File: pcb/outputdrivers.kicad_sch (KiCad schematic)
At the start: 15 parts, among them J7 CONTACTORS, J7 CP/PE, J7 RF, Q1 BC846, Q2 NCV8402xST, Q3 NCV8402xST, U7 74HCT04

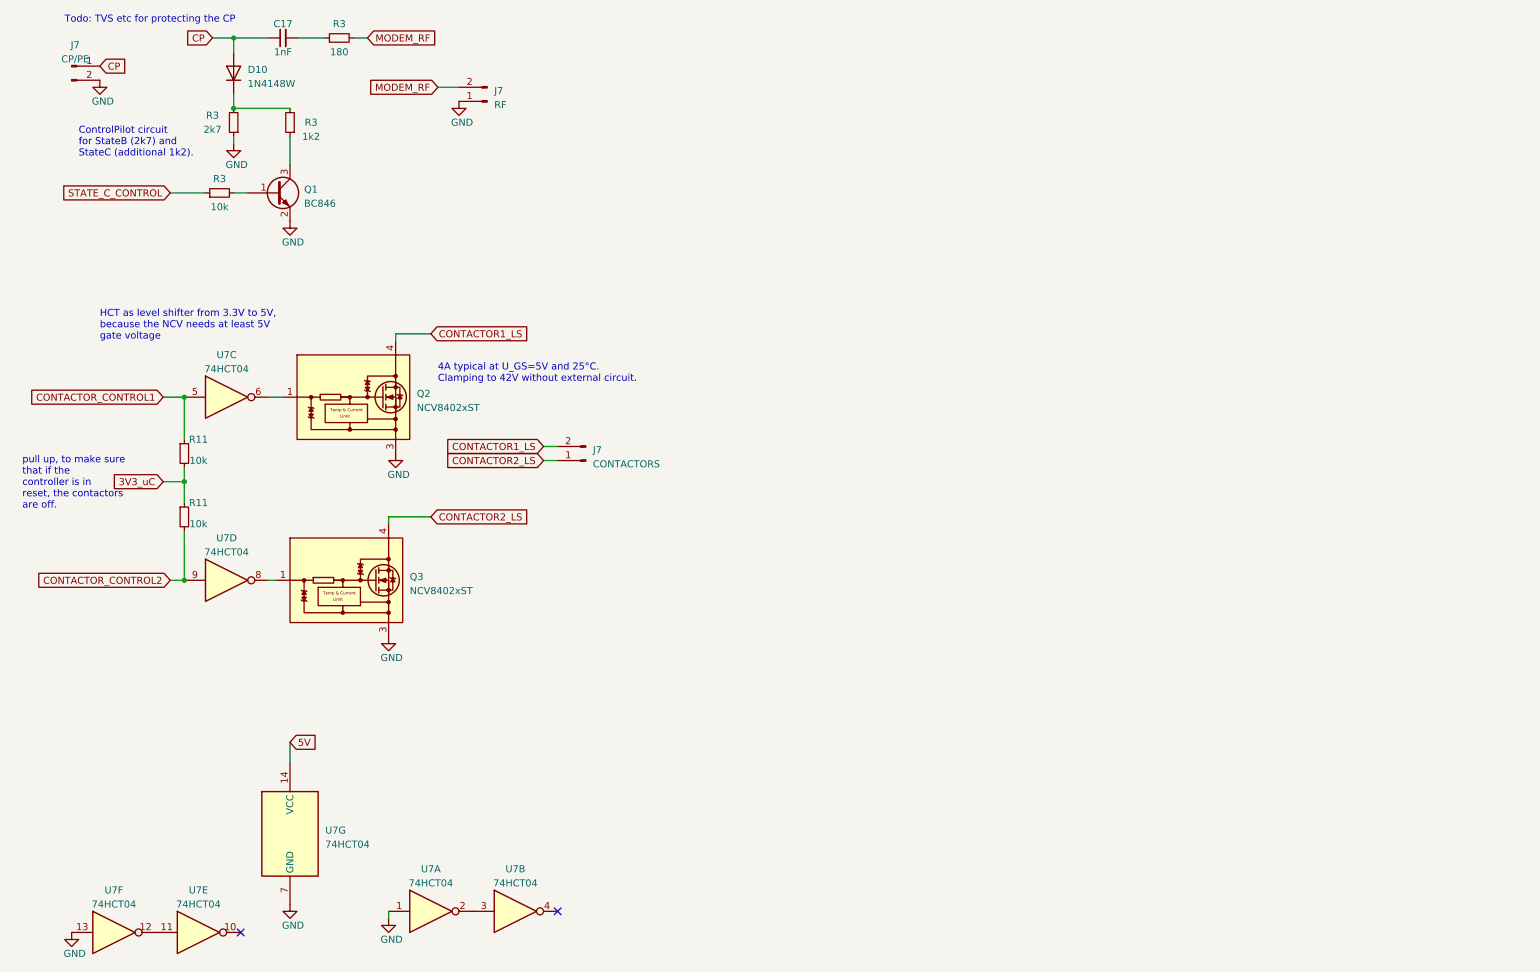
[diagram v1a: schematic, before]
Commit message: fix: divider on the stepdown. fix: non-inverted contactor drivers. fix: part number of 8MHz. add: mounting holes and spare grid. add: LIM HVDC input. docu: todo list
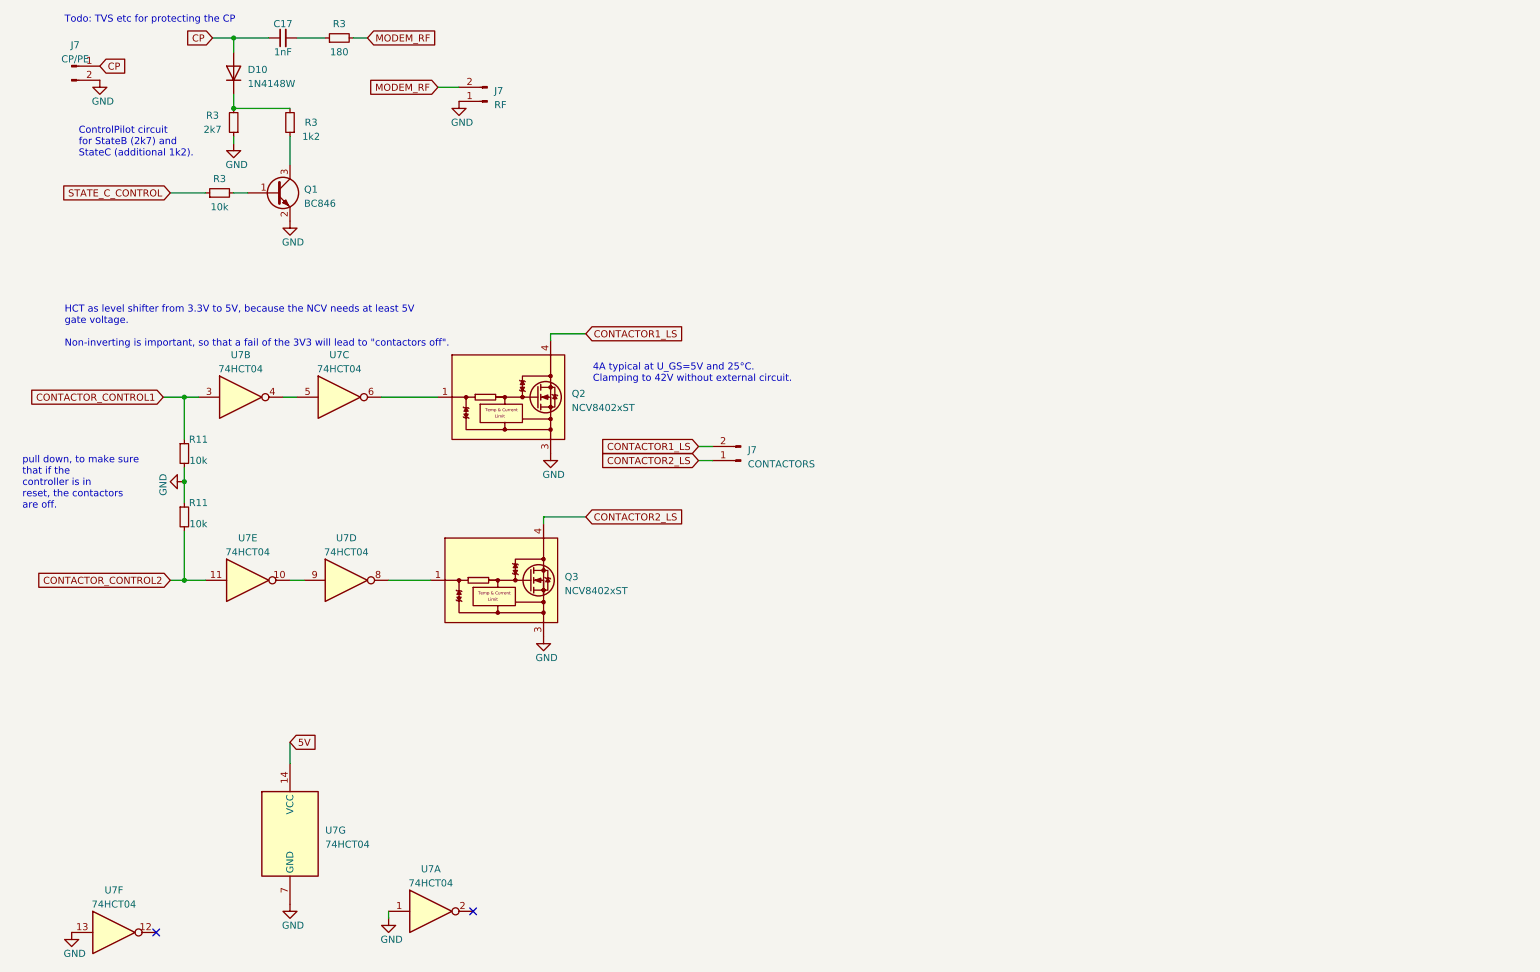
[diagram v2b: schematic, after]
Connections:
- net 3V3_uC is gone; now on net GND: R11.1, R11.2
- net CONTACTOR_CONTROL1: now also U7.3; no longer U7.5
- net CONTACTOR_CONTROL2: now also U7.11; no longer U7.9
- net at U7.2: no longer U7.3
- net at U7.12: no longer U7.11
- net at U7.10: now also U7.9
- net at U7.4: now also U7.5
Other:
- note added: "HCT as level shifter from 3.3V to 5V, because the NCV needs at least 5V gate voltage. Non-inverting is important, so that a fail of the 3V3 will lead to "contactors off"."
- note added: "pull down, to make sure that if the controller is in reset, the contactors are off."
- note removed: "HCT as level shifter from 3.3V to 5V, because the NCV needs at least 5V gate voltage"
- note removed: "pull up, to make sure that if the controller is in reset, the contactors are off."
- moved on the sheet: J7, Q2, Q3, U7B, U7C, U7D, U7E

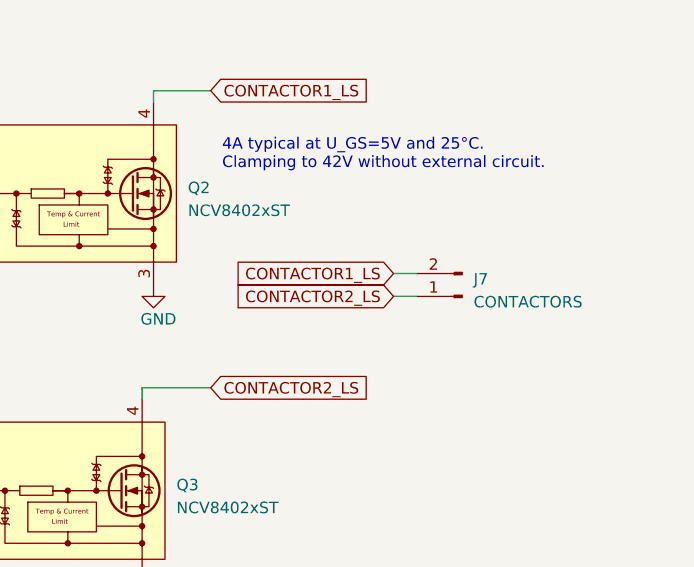
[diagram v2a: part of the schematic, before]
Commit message: added TE DEUTSCH connector and housing
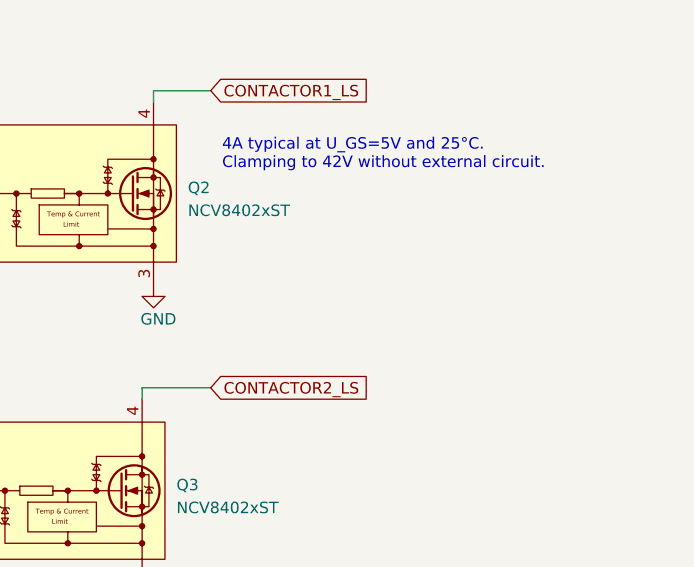
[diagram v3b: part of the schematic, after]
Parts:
- removed J7: CONTACTORS, Connector_PinHeader_2.54mm:PinHeader_1x02_P2.54mm_Vertical, symbol Connector:Conn_01x02_Pin
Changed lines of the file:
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@@
-    (stroke (width 0) (type default))
-  )
-  (wire (pts (xy 140.97 100.33) (xy 143.51 100.33))
     (stroke (width 0) (type default))
   )
@@
   )
   (wire (pts (xy 93.98 35.56) (xy 97.79 35.56))
-    (stroke (width 0) (type default))
-  )
-  (wire (pts (xy 140.97 102.87) (xy 143.51 102.87))
     (stroke (width 0) (type default))
   )
@@
     (at 121.92 88.9 0)
     (effects (font (size 1.27 1.27)) (justify left bottom))
-  )
-  (global_label "CONTACTOR1_LS" (shape input) (at 140.97 100.33 180) (fields_autoplaced)
-    (effects (font (size 1.27 1.27)) (justify right))
-    (property "Intersheetrefs" "${INTERSHEET_REFS}" (at 122.8242 100.33 0)
-      (effects (font (size 1.27 1.27)) (justify right) hide)
-    )
   )
   (global_label "5V" (shape input) (at 67.31 153.67 0) (fields_autoplaced)
@@
     (effects (font (size 1.27 1.27)) (justify right))
     (property "Intersheetrefs" "${INTERSHEET_REFS}" (at 81.0957 35.56 0)
-      (effects (font (size 1.27 1.27)) (justify right) hide)
-    )
-  )
-  (global_label "CONTACTOR2_LS" (shape input) (at 140.97 102.87 180) (fields_autoplaced)
-    (effects (font (size 1.27 1.27)) (justify right))
-    (property "Intersheetrefs" "${INTERSHEET_REFS}" (at 122.8242 102.87 0)
       (effects (font (size 1.27 1.27)) (justify right) hide)
     )
@@
         )
       )
-    )
-  )
-  (symbol (lib_id "Connector:Conn_01x02_Pin") (at 148.59 102.87 180) (unit 1)
-    (in_bom yes) (on_board yes) (dnp no) (fields_autoplaced)
-    (property "Reference" "J7" (at 149.86 100.965 0)
-      (effects (font (size 1.27 1.27)) (justify right))
-    )
-    (property "Value" "CONTACTORS" (at 149.86 103.505 0)
-      (effects (font (size 1.27 1.27)) (justify right))
-    )
-    (property "Footprint" "Connector_PinHeader_2.54mm:PinHeader_1x02_P2.54mm_Vertical" (at 148.59 102.87 0)
-      (effects (font (size 1.27 1.27)) hide)
-    )
-    (property "Datasheet" "~" (at 148.59 102.87 0)
-      (effects (font (size 1.27 1.27)) hide)
-    )
-    (pin "1")
-    (pin "2")
-    (instances
-      (project "qca7000"
-        (path "/e63e39d7-6ac0-4ffd-8aa3-1841a4541b55/5666e7cf-6b6c-4583-8335-aa3be69ccd45"
-          (reference "J7") (unit 1)
-        )
-        (path "/e63e39d7-6ac0-4ffd-8aa3-1841a4541b55/539ec63d-ac7e-42ea-858e-ff2bf33430ea"
-          (reference "J8") (unit 1)
-        )
-      )

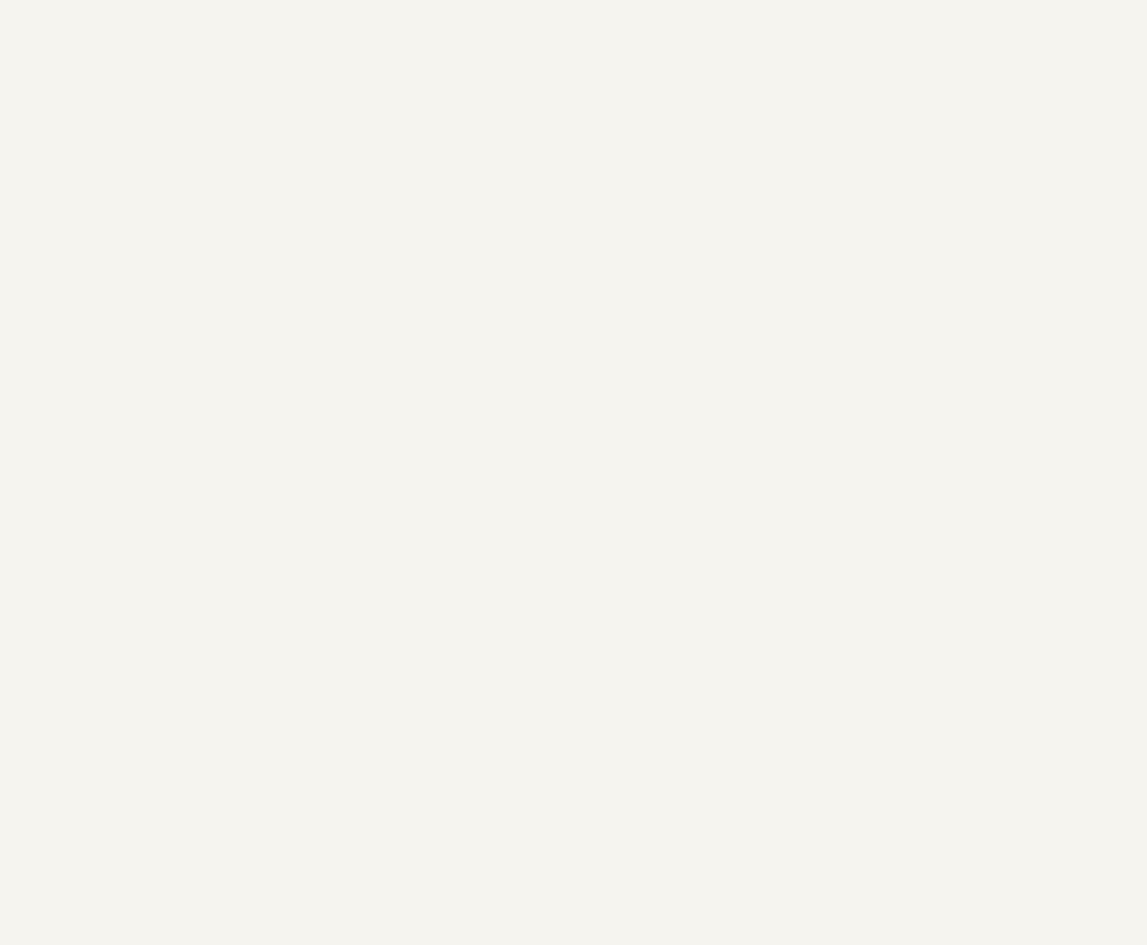
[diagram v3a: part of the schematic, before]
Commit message: added RGB LED highside drivers
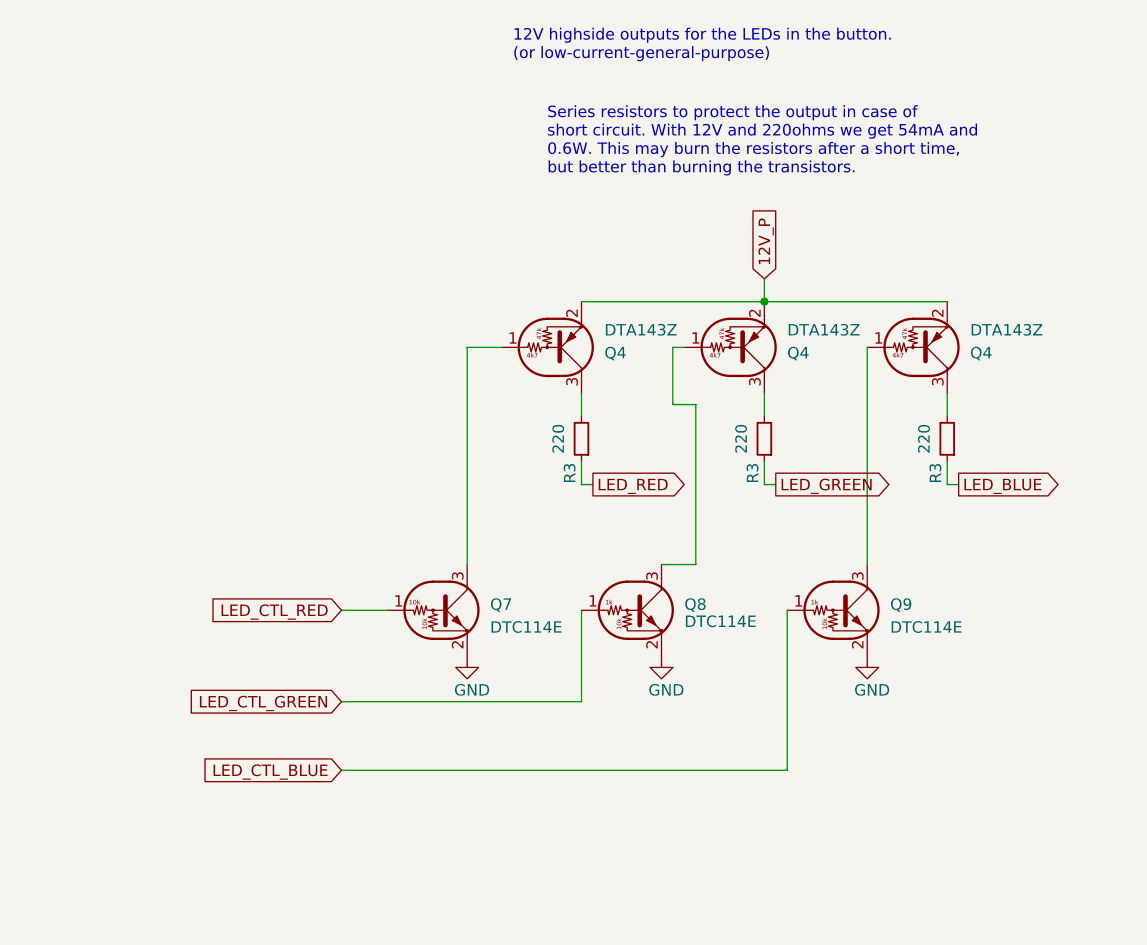
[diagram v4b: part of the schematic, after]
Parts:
- added Q4 (x3): DTA143Z, Package_TO_SOT_SMD:SOT-23, symbol Transistor_BJT:DTA143Z
- added Q7: DTC114E, Package_TO_SOT_SMD:SOT-23, symbol Transistor_BJT:DTC114E
- added Q8, Q9: DTC114E, Package_TO_SOT_SMD:SOT-23, symbol Transistor_BJT:DTC113Z
- added R3 (x3): 220, Resistor_SMD:R_1206_3216Metric_Pad1.30x1.75mm_HandSolder, symbol Device:R_Small
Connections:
- net GND: now also Q7.2 (E), Q8.2 (E), Q9.2 (E)
- new net: Q4.1 (B), Q7.3 (C)
- new net: Q4.1 (B), Q8.3 (C)
- new net: Q4.3 (C), R3.2 (x3)
- new net: Q4.1 (B), Q9.3 (C)
- new net 12V_P: Q4.2 (E), Q4.2 (E), Q4.2 (E)
- new net LED_BLUE: R3.1
- new net LED_CTL_BLUE: Q9.1 (B)
- new net LED_CTL_GREEN: Q8.1 (B)
- new net LED_CTL_RED: Q7.1 (B)
- new net LED_GREEN: R3.1
- new net LED_RED: R3.1
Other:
- note added: "12V highside outputs for the LEDs in the button. (or low-current-general-purpose)"
- note added: "Series resistors to protect the output in case of short circuit. With 12V and 220ohms we get 54mA and 0.6W. This may burn the resistors after a short time, but better than burning the transistors."
